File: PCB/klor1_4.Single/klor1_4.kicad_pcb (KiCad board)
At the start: 2 copper layers, 160 x 118.2 mm, 88 parts, among them J1 MJ-4PP-9, J2 Haptic Buzz, J3 lv27, SW1 SW_PUSH-MX_W_LED, SW10 SW_PUSH-MX_W_LED, SW11 SW_PUSH-MX_W_LED, SW12 SW_PUSH-MX_W_LED, SW13 SW_PUSH-MX_W_LED, SW14 SW_PUSH-MX_W_LED, SW15 SW_PUSH-MX_W_LED, SW16 SW_PUSH-MX_W_LED, SW17 SW_PUSH-MX_W_LED, SW18 RotaryEncoder_Switch, SW19 SW_PUSH-MX_W_LED, SW2 SW_PUSH-MX_W_LED, SW20 SW_PUSH-MX_W_LED, SW21 SW_PUSH-MX_W_LED, SW22 SW_PUSH-MX_W_LED, SW3 SW_PUSH-MX_W_LED, SW4 SW_PUSH-MX_W_LED, SW5 SW_PUSH-MX_W_LED, SW6 SW_PUSH-MX_W_LED, SW7 SW_PUSH-MX_W_LED, SW8 SW_PUSH-MX_W_LED, SW9 SW_PUSH-MX_W_LED, U1 ProMicro_Single

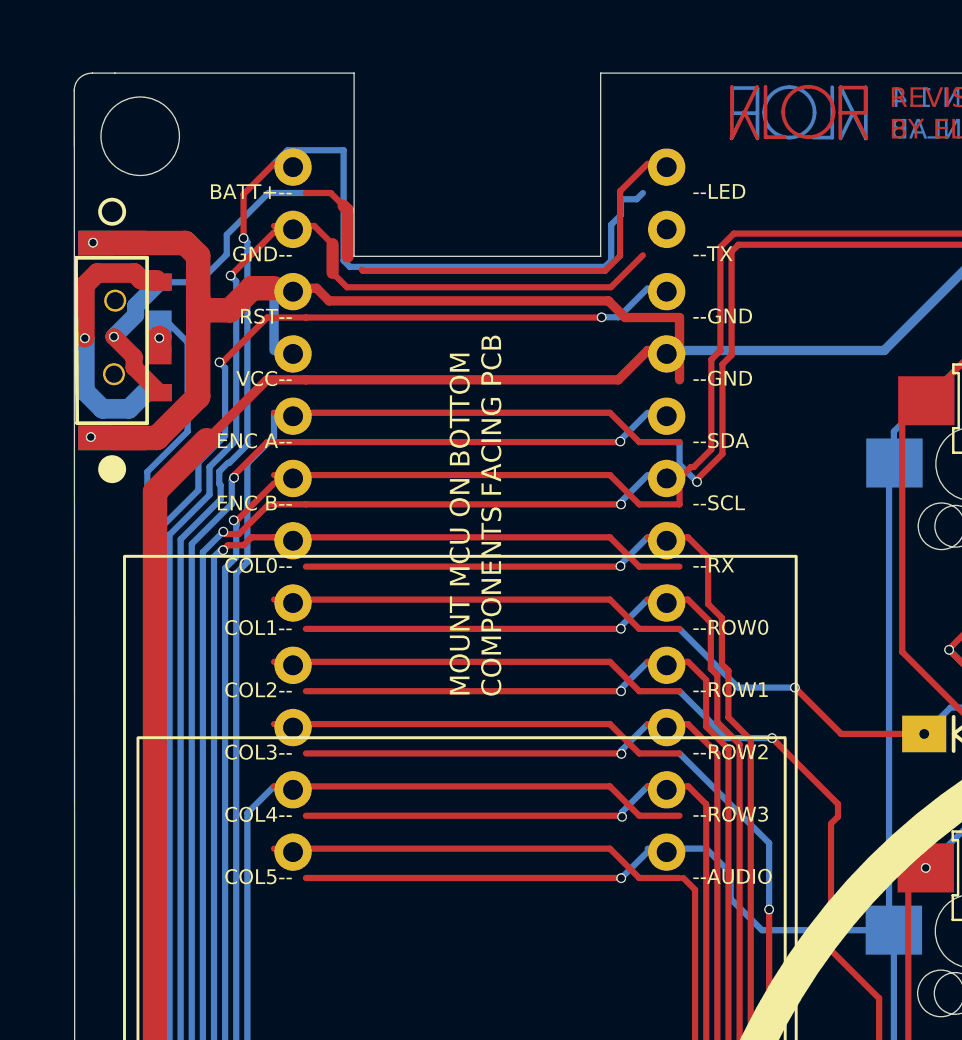
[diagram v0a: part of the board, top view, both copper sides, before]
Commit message: single 2504151724
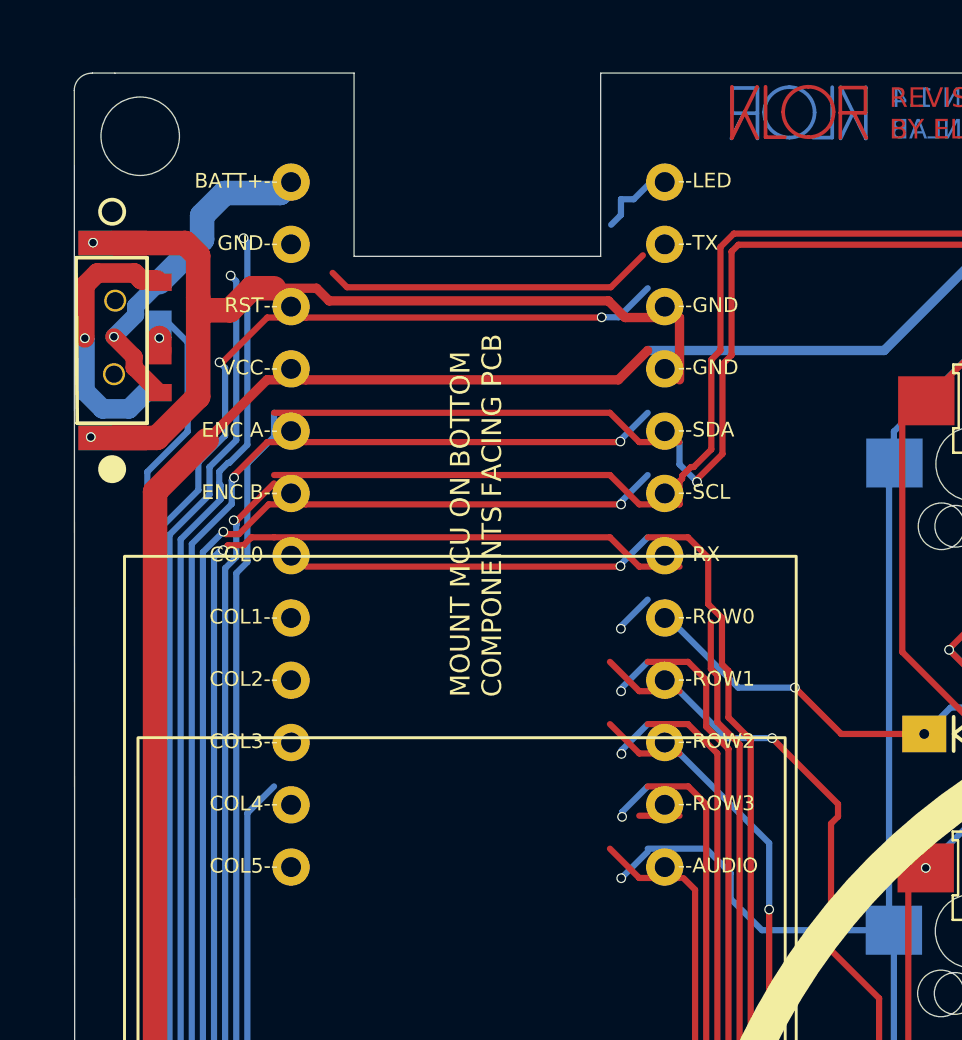
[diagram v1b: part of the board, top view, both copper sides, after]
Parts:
- moved U1 0.62 mm to (98.3, 72.4)
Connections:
- U1 pad 1: (no net) -> +BATT
- U1 pad 10: (no net) -> col3
- U1 pad 11: (no net) -> col4
- U1 pad 12: (no net) -> col5
- U1 pad 13: (no net) -> AUDIO
- U1 pad 14: (no net) -> row3
- U1 pad 15: (no net) -> row2
- U1 pad 16: (no net) -> row1
- U1 pad 17: (no net) -> row0
- U1 pad 18: (no net) -> RX
- U1 pad 19: (no net) -> SCL
- U1 pad 2: (no net) -> GND
- U1 pad 20: (no net) -> SDA
- U1 pad 21: (no net) -> GND
- U1 pad 22: (no net) -> GND
- U1 pad 3: (no net) -> RESET
- U1 pad 4: (no net) -> VCC
- U1 pad 5: (no net) -> ENCA
- U1 pad 6: (no net) -> ENCB
- U1 pad 7: (no net) -> col0
- U1 pad 8: (no net) -> col1
- U1 pad 9: (no net) -> col2
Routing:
- net LED: track 172.8 -> 135.6 mm
- net row0: track 126.1 -> 109.0 mm
- net row3: track 168.6 -> 151.6 mm
- net col1: track 294.6 -> 278.8 mm
- net row1: track 176.3 -> 162.6 mm
- net row2: track 193.6 -> 179.9 mm
- net AUDIO: track 103.2 -> 89.5 mm
- net col5: track 141.9 -> 129.0 mm
- net col2: track 261.9 -> 249.0 mm
- net col3: track 255.3 -> 242.4 mm
- net col4: track 256.1 -> 244.9 mm
- net TX: track 92.2 -> 85.8 mm
- net +BATT: track 17.9 -> 13.7 mm
- net GND: track 195.7 -> 193.2 mm
